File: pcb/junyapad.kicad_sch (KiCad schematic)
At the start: 40 parts, among them J1 OLED_128x32, SW1 SW_Push_45deg, SW2 SW_Push_45deg, SW3 SW_Push_45deg, SW4 SW_Push_45deg, SW5 SW_Push_45deg, SW6 SW_Push_45deg, SW7 SW_Push_45deg, SW8 SW_Push_45deg, SW9 RotaryEncoder_Switch, U1 XIAO-RP2040-DIP

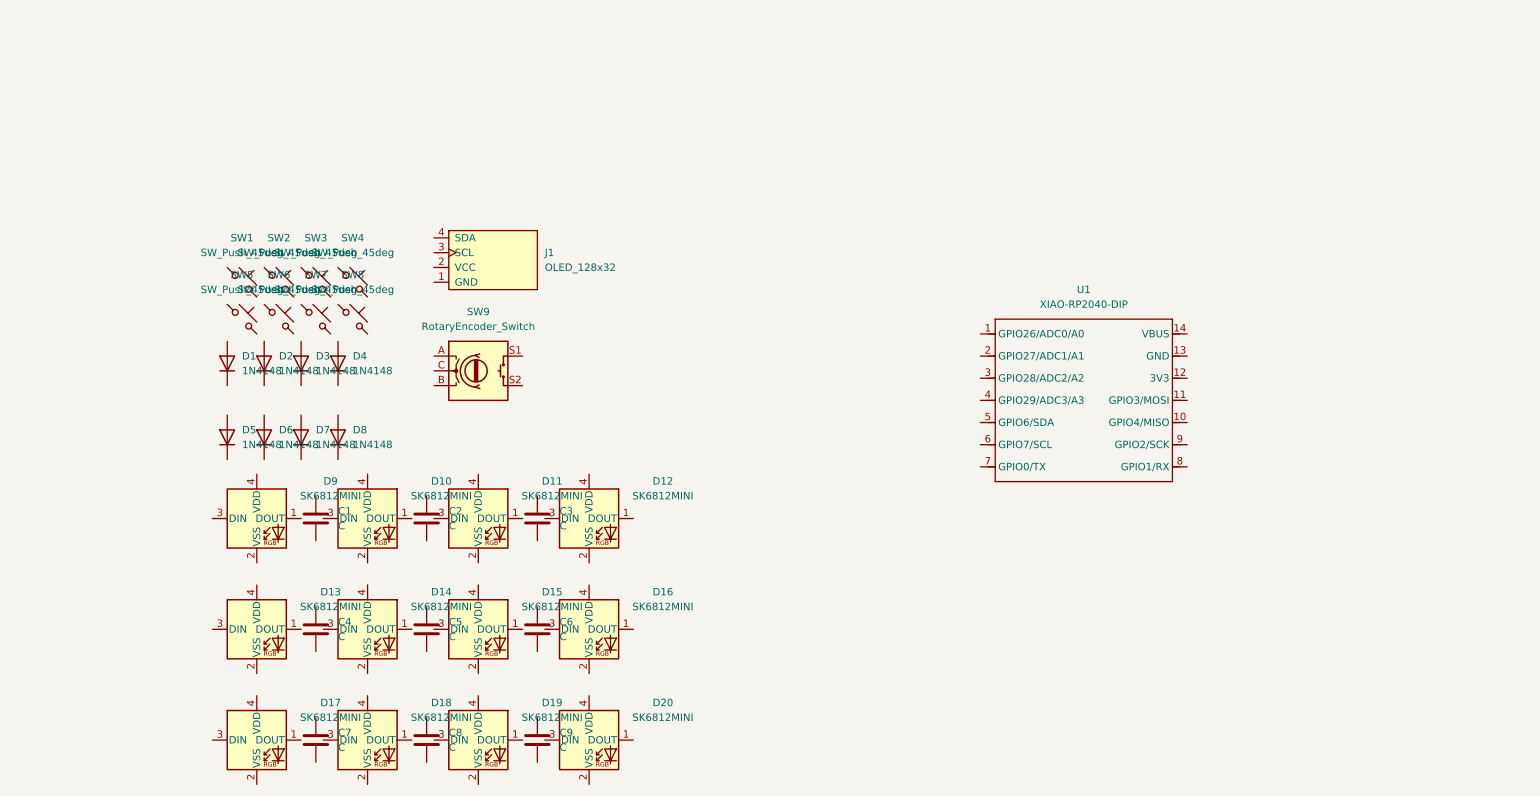
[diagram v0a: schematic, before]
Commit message: Update schematic
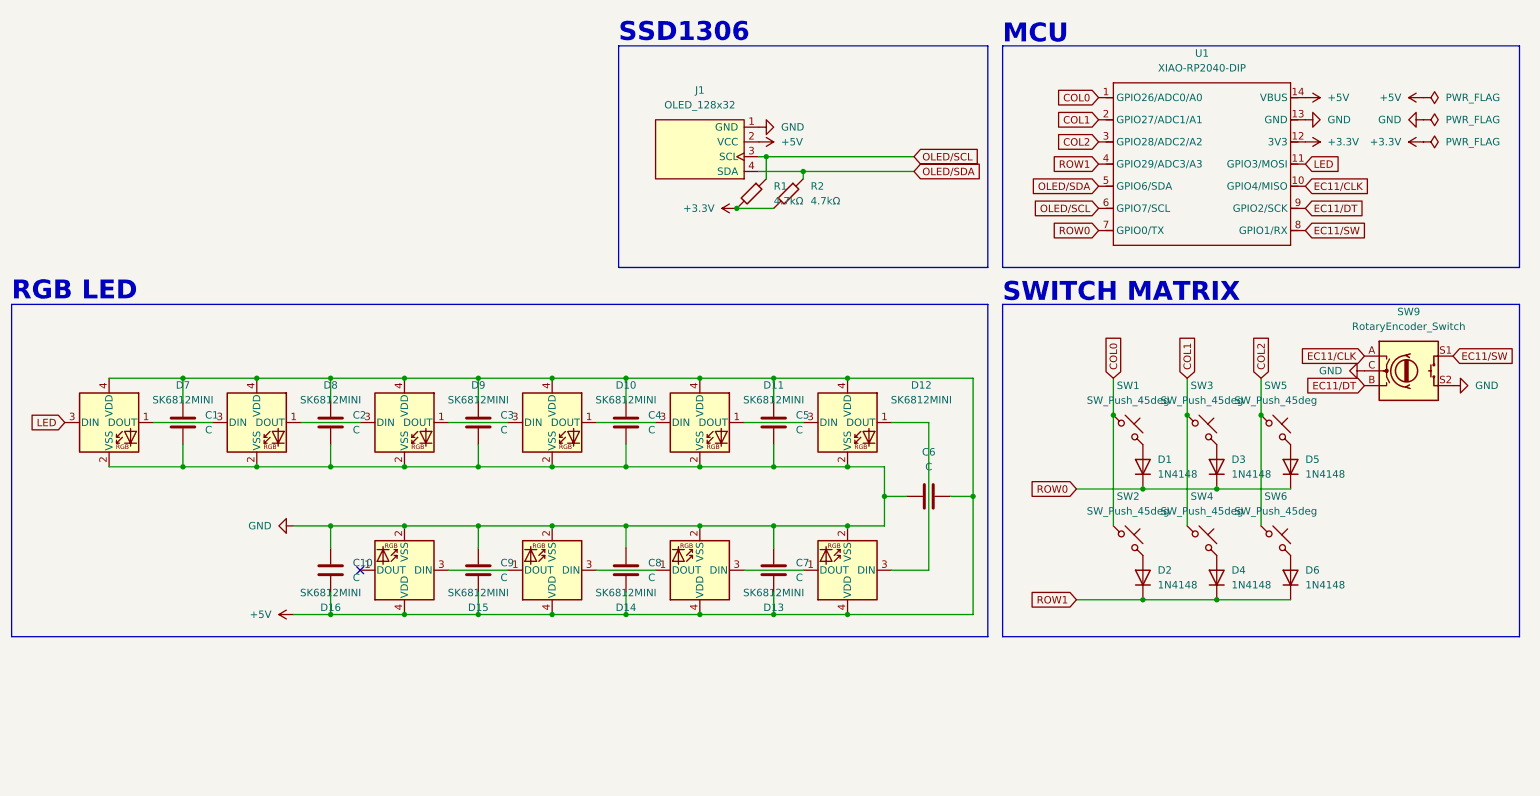
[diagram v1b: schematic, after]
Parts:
- removed D17, D18, D19, D20: SK6812MINI, LED_SMD:LED_SK6812MINI_PLCC4_3.5x3.5mm_P1.75mm, symbol LED:SK6812MINI
- removed D7, D8: 1N4148, Diode_THT:D_DO-35_SOD27_P7.62mm_Horizontal, symbol Diode:1N4148
- removed SW7, SW8: SW_Push_45deg, symbol Switch:SW_Push_45deg
- added C10: C, Capacitor_THT:C_Disc_D3.0mm_W1.6mm_P2.50mm, symbol Device:C
- added D7, D8: SK6812MINI, LED_SMD:LED_SK6812MINI_PLCC4_3.5x3.5mm_P1.75mm, symbol LED:SK6812MINI
- added R1, R2: 4.7kΩ, Resistor_THT:R_Axial_DIN0204_L3.6mm_D1.6mm_P7.62mm_Horizontal, symbol Device:R_45deg
- C1, C2, C3, C4, C5, C6, C7, C8, C9: footprint (none) -> Capacitor_THT:C_Disc_D3.0mm_W1.6mm_P2.50mm
- SW1, SW2, SW3, SW4, SW5, SW6: footprint (none) -> MX_Solderable:MX-Solderable-1U
- SW9: footprint (none) -> Rotary_Encoder:RotaryEncoder_Alps_EC11E-Switch_Vertical_H20mm
- U1: footprint Module:MOUDLE14P-XIAO-DIP-SMD -> OPL:XIAO-RP2040-DIP
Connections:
- net EC11/CLK: now reaches SW9.A
- net EC11/CLK: now also U1.10 (GPIO4/MISO)
- net EC11/DT: now reaches SW9.B
- net EC11/DT: now also U1.9 (GPIO2/SCK)
- net GND: now reaches SW9.C
- net GND: now also C1.2, C2.2, C3.2, C4.2, C5.2, C6.1, C7.1, C8.1, C9.1, D10.2 (VSS), D11.2 (VSS), D12.2 (VSS), D13.2 (VSS), D14.2 (VSS), D15.2 (VSS), D16.2 (VSS), D9.2 (VSS), J1.1 (GND), SW9.S2, U1.13 (GND), C10.1, D7.2 (VSS), D8.2 (VSS)
- net EC11/SW: now reaches SW9.S1
- net EC11/SW: now also U1.8 (GPIO1/RX)
- net COL2: now reaches SW5.1
- net COL2: now also SW6.1, U1.3 (GPIO28/ADC2/A2)
- net at SW5.2: now also D5.2 (A)
- net at D12.1 (DOUT): now also D13.3 (DIN)
- net at D12.3 (DIN): now also D11.1 (DOUT)
- net +5V: now reaches D12.4 (VDD)
- net +5V: now also C1.1, C2.1, C3.1, C4.1, C5.1, C6.2, C7.2, C8.2, C9.2, D10.4 (VDD), D11.4 (VDD), D13.4 (VDD), D14.4 (VDD), D15.4 (VDD), D16.4 (VDD), D9.4 (VDD), J1.2 (VCC), U1.14 (VBUS), C10.2, D7.4 (VDD), D8.4 (VDD)
- net ROW0: now reaches D5.1 (K)
- net ROW0: now also D1.1 (K), D3.1 (K), U1.7 (GPIO0/TX)
- net COL0: now reaches SW1.1
- net COL0: now also SW2.1, U1.1 (GPIO26/ADC0/A0)
- net at SW1.2: now also D1.2 (A)
- net at D11.3 (DIN): now also D10.1 (DOUT)
- net at SW6.2: now also D6.2 (A)
- net ROW1: now reaches D2.1 (K)
- net ROW1: now also D4.1 (K), D6.1 (K), U1.4 (GPIO29/ADC3/A3)
- net at D2.2 (A): now also SW2.2
- net at D15.1 (DOUT): now also D16.3 (DIN)
- net at D15.3 (DIN): now also D14.1 (DOUT)
- net at D10.3 (DIN): now also D9.1 (DOUT)
- net COL1: now reaches SW3.1
- net COL1: now also SW4.1, U1.2 (GPIO27/ADC1/A1)
- net at SW3.2: now also D3.2 (A)
- net at D4.2 (A): now also SW4.2
- net at D14.3 (DIN): now also D13.1 (DOUT)
- net at D9.3 (DIN): now also D8.1 (DOUT)
- net LED: now reaches U1.11 (GPIO3/MOSI)
- net LED: now also D7.3 (DIN)
- net +3.3V: now reaches U1.12 (3V3)
- net +3.3V: now also R1.2, R2.2
- net OLED/SDA: now reaches U1.5 (GPIO6/SDA)
- net OLED/SDA: now also J1.4 (SDA), R2.1
- net OLED/SCL: now reaches U1.6 (GPIO7/SCL)
- net OLED/SCL: now also J1.3 (SCL), R1.1
- new net: D7.1 (DOUT), D8.3 (DIN)
- no-connect marks 0 -> 1
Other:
- note added: "MCU"
- note added: "RGB LED"
- note added: "SSD1306"
- note added: "SWITCH MATRIX"
- moved on the sheet: D1, D2, D3, D4, D5, D6, J1, SW1, SW2, SW3, SW4, SW5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
